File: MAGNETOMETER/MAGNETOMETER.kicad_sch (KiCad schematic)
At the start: 5 parts, among them IC6 MMC5603NJ, J1 M80-8770405

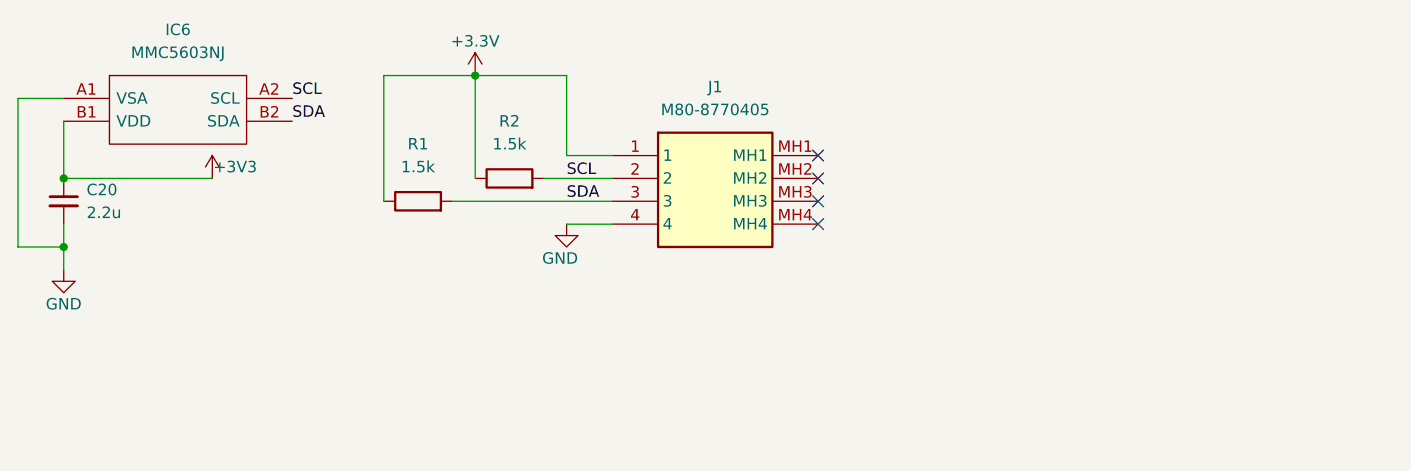
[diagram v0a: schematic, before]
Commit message: LC24 PCBs
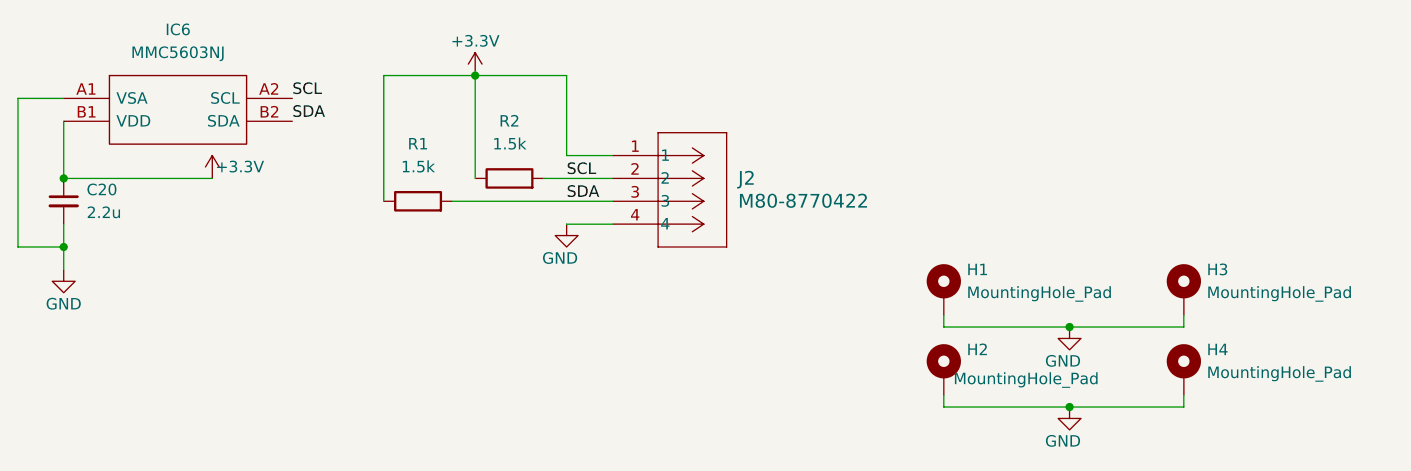
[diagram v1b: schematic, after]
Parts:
- removed J1: M80-8770405, M808770405, symbol M80-8770405:M80-8770405
- added H1, H2, H3, H4: MountingHole_Pad, Mounting_Wuerth:Mounting_Wuerth_WA-SMSI-M1.6_H1mm_9774010633, symbol Mechanical:MountingHole_Pad
- added J2: M80-8770422, Harwin-M80-8770422:CONN_M80-87704_HRW, symbol Harwin-M80-8770422:M80-8770422
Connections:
- net +3V3 is gone; now on net +3.3V: C20.1, IC6.B1 (VDD)
- net +3.3V: now also J2.1
- net GND: now also H1.1, H2.1, H3.1, H4.1, J2.4
- net SCL: now also J2.2
- net SDA: now also J2.3
- no-connect marks 4 -> 0
